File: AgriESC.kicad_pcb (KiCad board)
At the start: 2 copper layers, 91.9 x 64 mm, 312 parts, among them J1 SUPPLY, J10 GPIO, J11 USB_OTG, J12 HALL_ENC, J2 PH_A, J3 PH_B, J4 PH_C, J6 COMM, J7 SERVO, J8 CAN, J9 SWD, SW1 SW_SPDT, U1 FDMS7698, U10 STM32F405RGT6, U11 DRV8303, U12 TJA1051TK-3, U13 LMR16006YQ, U14 MCP1700-3302E_SOT23, U15 MCP1700-3302E_SOT23, U2 FDMS7698, U3 FDMS7698, U4 FDMS7698, U5 FDMS7698, U6 FDMS7698, U7 MAX9920, U8 MAX9920, U9 MAX9920, Y1 8M Resonator

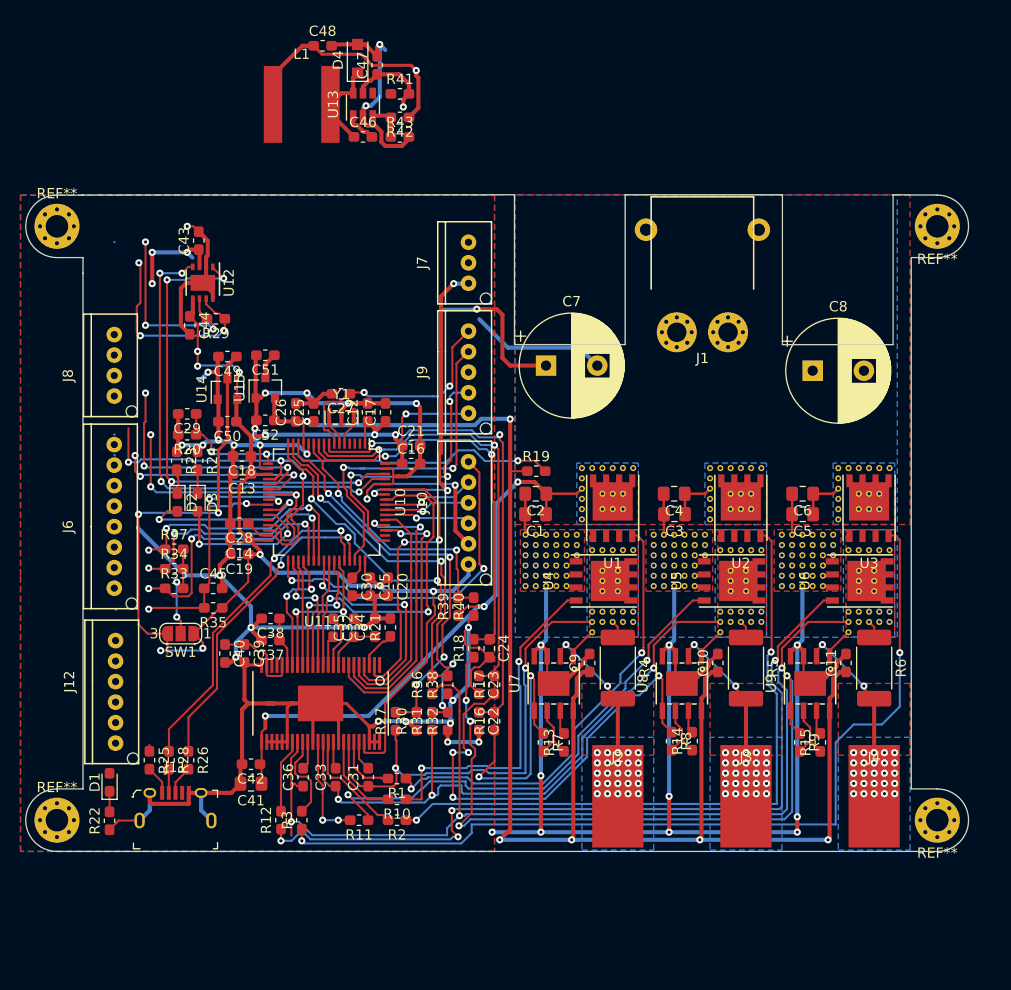
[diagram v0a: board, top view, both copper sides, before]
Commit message: Version 1.0 completed
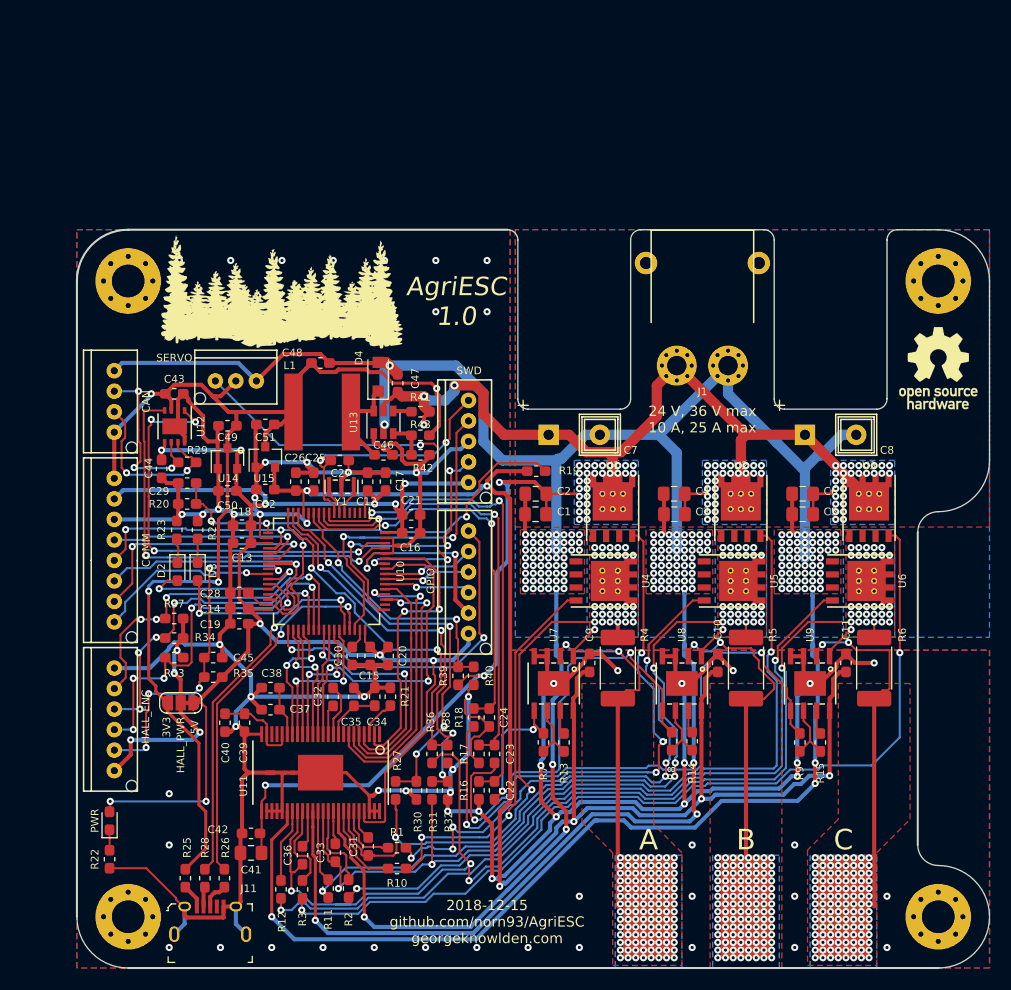
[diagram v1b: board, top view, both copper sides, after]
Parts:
- removed D1: BLUE, LED_SMD:LED_0603_1608Metric_Pad1.05x0.95mm_HandSolder
- removed J10: GPIO, AgriESC:JST_PA_01x06
- removed J12: HALL_ENC, AgriESC:JST_PA_01x06
- removed J4: PH_C, Connector_Wire:SolderWirePad_1x01_SMD_5x10mm
- removed J6: COMM, AgriESC:JST_PA_01x08
- removed J7: SERVO, AgriESC:JST_PA_01x03
- removed J8: CAN, AgriESC:JST_PA_01x04
- removed J9: SWD, AgriESC:JST_PA_01x05
- removed the REF** at (194.9, 64.7)
- removed the REF** at (188.2, 103.2)
- removed the REF** at (172.8, 91.2)
- removed the REF** at (172.8, 90.2)
- removed the REF** at (172.8, 89.2)
- removed the REF** at (172.8, 88.2)
- removed the REF** at (173.8, 88.2)
- removed the REF** at (174.8, 88.2)
- removed the REF** at (175.8, 88.2)
- removed the REF** at (176.8, 88.2)
- removed the REF** at (177.8, 88.2)
- removed the REF** at (177.8, 103.2)
- removed the REF** at (188.2, 102.2)
- removed the REF** at (176.8, 103.2)
- removed the REF** at (175.8, 103.2)
- removed the REF** at (174.8, 103.2)
- removed the REF** at (173.8, 104.2)
- removed the REF** at (173.8, 103.2)
- removed the REF** at (173.8, 102.2)
- removed the REF** at (174.8, 102.2)
- removed the REF** at (175.8, 102.2)
- removed the REF** at (176.8, 102.2)
- removed the REF** at (177.8, 102.2)
- removed the REF** at (189.2, 103.2)
- removed the REF** at (177.8, 96.2)
- removed the REF** at (176.8, 96.2)
- removed the REF** at (175.8, 96.2)
- removed the REF** at (174.8, 96.2)
- removed the REF** at (173.8, 96.2)
- removed the REF** at (165.2, 88.2)
- removed the REF** at (164.2, 88.2)
- removed the REF** at (163.2, 88.2)
- removed the REF** at (162.2, 88.2)
- removed the REF** at (161.2, 88.2)
- removed the REF** at (189.2, 102.2)
- removed the REF** at (160.2, 88.2)
- removed the REF** at (160.2, 89.2)
- removed the REF** at (160.2, 90.2)
- removed the REF** at (160.2, 91.2)
- removed the REF** at (160.2, 92.2)
- removed the REF** at (160.2, 93.2)
- removed the REF** at (158.8, 99.8)
- removed the REF** at (157.8, 99.8)
- removed the REF** at (156.8, 99.8)
- removed the REF** at (155.8, 99.8)
- removed the REF** at (190.2, 103.2)
- removed the REF** at (154.8, 99.8)
- removed the REF** at (158.8, 98.8)
- removed the REF** at (157.8, 98.8)
- removed the REF** at (156.8, 98.8)
- removed the REF** at (155.8, 98.8)
- removed the REF** at (154.8, 98.8)
- removed the REF** at (158.8, 97.8)
- removed the REF** at (157.8, 97.8)
- removed the REF** at (156.8, 97.8)
- removed the REF** at (155.8, 97.8)
- removed the REF** at (190.2, 102.2)
- removed the REF** at (154.8, 97.8)
- removed the REF** at (158.8, 96.8)
- removed the REF** at (157.8, 96.8)
- removed the REF** at (156.8, 96.8)
- removed the REF** at (155.8, 96.8)
- removed the REF** at (154.8, 96.8)
- removed the REF** at (159.8, 95.8)
- removed the REF** at (158.8, 95.8)
- removed the REF** at (157.8, 95.8)
- removed the REF** at (156.8, 95.8)
- removed the REF** at (190.2, 96.2)
- removed the REF** at (155.8, 95.8)
- removed the REF** at (154.8, 95.8)
- removed the REF** at (159.8, 94.8)
- removed the REF** at (158.8, 94.8)
- removed the REF** at (157.8, 94.8)
- removed the REF** at (156.8, 94.8)
- removed the REF** at (155.8, 94.8)
- removed the REF** at (154.8, 94.8)
- removed the REF** at (165.2, 103.2)
- removed the REF** at (164.2, 103.2)
- removed the REF** at (189.2, 96.2)
- removed the REF** at (163.2, 103.2)
- removed the REF** at (162.2, 103.2)
- removed the REF** at (161.2, 104.2)
- removed the REF** at (161.2, 103.2)
- removed the REF** at (161.2, 102.2)
- removed the REF** at (165.2, 102.2)
- removed the REF** at (164.2, 102.2)
- removed the REF** at (163.2, 102.2)
- removed the REF** at (162.2, 102.2)
- removed the REF** at (165.2, 96.2)
- removed the REF** at (188.2, 96.2)
- removed the REF** at (164.2, 96.2)
- removed the REF** at (163.2, 96.2)
- removed the REF** at (162.2, 96.2)
- removed the REF** at (161.2, 96.2)
- removed the REF** at (109.1, 64.7)
- removed the REF** at (187.2, 96.2)
- removed the REF** at (194.9, 122.6)
- removed the REF** at (186.2, 96.2)
- removed the REF** at (190.2, 88.2)
- removed the REF** at (189.2, 88.2)
- removed the REF** at (188.2, 88.2)
- removed the REF** at (187.2, 88.2)
- removed the REF** at (186.2, 88.2)
- removed the REF** at (185.2, 93.2)
- removed the REF** at (185.2, 92.2)
- removed the REF** at (185.2, 91.2)
- removed the REF** at (185.2, 90.2)
- removed the REF** at (109.1, 122.6)
- removed the REF** at (185.2, 89.2)
- removed the REF** at (185.2, 88.2)
- removed the REF** at (183.8, 99.8)
- removed the REF** at (182.8, 99.8)
- removed the REF** at (181.8, 99.8)
- removed the REF** at (180.8, 99.8)
- removed the REF** at (179.8, 99.8)
- removed the REF** at (183.8, 98.8)
- removed the REF** at (182.8, 98.8)
- removed the REF** at (181.8, 98.8)
- removed the REF** at (159.8, 96.8)
- removed the REF** at (180.8, 98.8)
- removed the REF** at (179.8, 98.8)
- removed the REF** at (183.8, 97.8)
- removed the REF** at (182.8, 97.8)
- removed the REF** at (181.8, 97.8)
- removed the REF** at (180.8, 97.8)
- removed the REF** at (179.8, 97.8)
- removed the REF** at (184.8, 96.8)
- removed the REF** at (183.8, 96.8)
- removed the REF** at (182.8, 96.8)
- removed the REF** at (186.2, 104.2)
- removed the REF** at (181.8, 96.8)
- removed the REF** at (180.8, 96.8)
- removed the REF** at (179.8, 96.8)
- removed the REF** at (184.8, 95.8)
- removed the REF** at (183.8, 95.8)
- removed the REF** at (182.8, 95.8)
- removed the REF** at (181.8, 95.8)
- removed the REF** at (180.8, 95.8)
- removed the REF** at (179.8, 95.8)
- removed the REF** at (184.8, 94.8)
- removed the REF** at (186.2, 103.2)
- removed the REF** at (183.8, 94.8)
- removed the REF** at (182.8, 94.8)
- removed the REF** at (181.8, 94.8)
- removed the REF** at (180.8, 94.8)
- removed the REF** at (179.8, 94.8)
- removed the REF** at (171.2, 99.8)
- removed the REF** at (170.2, 99.8)
- removed the REF** at (169.2, 99.8)
- removed the REF** at (168.2, 99.8)
- removed the REF** at (167.2, 99.8)
- removed the REF** at (186.2, 102.2)
- removed the REF** at (171.2, 98.8)
- removed the REF** at (170.2, 98.8)
- removed the REF** at (169.2, 98.8)
- removed the REF** at (168.2, 98.8)
- removed the REF** at (167.2, 98.8)
- removed the REF** at (171.2, 97.8)
- removed the REF** at (170.2, 97.8)
- removed the REF** at (169.2, 97.8)
- removed the REF** at (168.2, 97.8)
- removed the REF** at (167.2, 97.8)
- removed the REF** at (187.2, 103.2)
- removed the REF** at (172.2, 96.8)
- removed the REF** at (171.2, 96.8)
- removed the REF** at (170.2, 96.8)
- removed the REF** at (169.2, 96.8)
- removed the REF** at (168.2, 96.8)
- removed the REF** at (167.2, 96.8)
- removed the REF** at (172.2, 95.8)
- removed the REF** at (171.2, 95.8)
- removed the REF** at (170.2, 95.8)
- removed the REF** at (169.2, 95.8)
- removed the REF** at (187.2, 102.2)
- removed the REF** at (168.2, 95.8)
- removed the REF** at (167.2, 95.8)
- removed the REF** at (172.2, 94.8)
- removed the REF** at (171.2, 94.8)
- removed the REF** at (170.2, 94.8)
- removed the REF** at (169.2, 94.8)
- removed the REF** at (168.2, 94.8)
- removed the REF** at (167.2, 94.8)
- removed the REF** at (172.8, 93.2)
- removed the REF** at (172.8, 92.2)
- removed SW1: SW_SPDT, Jumper:SolderJumper-3_P1.3mm_Open_RoundedPad1.0x1.5mm_NumberLabels
- added C: PH_C, Connector_Wire:SolderWirePad_1x01_SMD_5x10mm, F.Cu at (185.8, 131.0)
- added CAN: CAN, AgriESC:JST_PA_01x04, F.Cu at (114.6, 82.8)
- added COMM: COMM, AgriESC:JST_PA_01x08, F.Cu at (114.6, 97.2)
- added G***: LOGO3, AgriESC:LOGO3, F.Cu at (131.0, 71.0)
- added GPIO: GPIO, AgriESC:JST_PA_01x06, F.Cu at (149.2, 98.4)
- added HALL_ENC: HALL_ENC, AgriESC:JST_PA_01x06, F.Cu at (114.7, 111.8)
- added HALL_PWR: SW_SPDT, Jumper:SolderJumper-3_P1.3mm_Open_RoundedPad1.0x1.5mm_NumberLabels, F.Cu at (121.1, 111.1)
- added NT1: Net-Tie_2, NetTie:NetTie-2_SMD_Pad0.5mm, B.Cu at (157.8, 106.0)
- added NT2: Net-Tie_2, NetTie:NetTie-2_SMD_Pad0.5mm, B.Cu at (170.2, 106.0)
- added NT3: Net-Tie_2, NetTie:NetTie-2_SMD_Pad0.5mm, B.Cu at (182.8, 106.0)
- added PWR: BLUE, LED_SMD:LED_0603_1608Metric_Pad1.05x0.95mm_HandSolder, F.Cu at (114.2, 122.6)
- added REF**: MountingHole_3.2mm_M3_Pad_Via, MountingHole:MountingHole_3.2mm_M3_Pad_Via, F.Cu at (116.0, 132.0)
- added REF**: MountingHole_3.2mm_M3_Pad_Via, MountingHole:MountingHole_3.2mm_M3_Pad_Via, F.Cu at (195.0, 70.0)
- added REF**: MountingHole_3.2mm_M3_Pad_Via, MountingHole:MountingHole_3.2mm_M3_Pad_Via, F.Cu at (195.0, 132.0)
- added REF**: MountingHole_3.2mm_M3_Pad_Via, MountingHole:MountingHole_3.2mm_M3_Pad_Via, F.Cu at (116.0, 70.0)
- added REF**: OSHW-Logo_7.5x8mm_SilkScreen, Symbol:OSHW-Logo_7.5x8mm_SilkScreen, F.Cu at (195.0, 78.5)
- added SERVO: SERVO, AgriESC:JST_PA_01x03, F.Cu at (126.5, 79.8)
- added SWD: SWD, AgriESC:JST_PA_01x05, F.Cu at (149.2, 85.6)
- C7, C8: footprint Capacitor_THT:CP_Radial_D10.0mm_P5.00mm -> AgriESC:CP_Radial_D10.0mm_P5.00mm_Side_Mounted
- moved U13 31.1 mm to (140.9, 83.8)
- moved C46 31.1 mm to (140.9, 87.0)
- moved C47 31.1 mm to (142.3, 80.0)
- moved D4 31.1 mm to (140.4, 79.3)
- moved R41 31.1 mm to (144.5, 82.8)
- moved R42 31.1 mm to (144.5, 85.0)
- moved R43 31.1 mm to (144.5, 87.0)
- moved C48 30.9 mm to (134.8, 78.0)
- moved L1 30.1 mm to (134.9, 82.8)
- moved C43 15.1 mm to (120.5, 81.0), turned to 0 degrees
- moved R29 14.3 mm to (121.8, 87.7)
- moved C44 14.3 mm to (119.3, 88.3)
- moved U12 14.3 mm to (120.5, 84.2)
- moved R25 12.0 mm to (121.6, 128.2)
- moved R26 12.0 mm to (125.4, 128.2)
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- renumbered J2 to A, J3 to B
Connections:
- C1 pad 2: SL_A -> GND
- C10 pad 2: SL_A -> GND
- C11 pad 2: SL_A -> GND
- C12 pad 2: SL_A -> GND
- C13 pad 2: SL_A -> GND
- C14 pad 2: SL_A -> GND
- C15 pad 2: SL_A -> GND
- C16 pad 2: SL_A -> GND
- C17 pad 2: SL_A -> GND
- C18 pad 2: SL_A -> GND
- C19 pad 2: SL_A -> GND
- C2 pad 2: SL_A -> GND
- C20 pad 2: SL_A -> GND
- C21 pad 2: SL_A -> GND
- C22 pad 2: SL_A -> GND
- C23 pad 2: SL_A -> GND
- C24 pad 2: SL_A -> GND
- C25 pad 2: SL_A -> GND
- C26 pad 2: SL_A -> GND
- C27 pad 2: SL_A -> GND
- C28 pad 2: SL_A -> GND
- C29 pad 2: SL_A -> GND
- C3 pad 2: SL_A -> GND
- C30 pad 2: SL_A -> GND
- C34 pad 2: SL_A -> GND
- C35 pad 2: SL_A -> GND
- C37 pad 2: SL_A -> GND
- C38 pad 2: SL_A -> GND
- C39 pad 2: SL_A -> GND
- C4 pad 2: SL_A -> GND
- C40 pad 2: SL_A -> GND
- C41 pad 2: SL_A -> GND
- C42 pad 2: SL_A -> GND
- C43 pad 2: SL_A -> GND
- C44 pad 2: SL_A -> GND
- C45 pad 2: SL_A -> GND
- C47 pad 2: SL_A -> GND
- C48 pad 2: SL_A -> GND
- C49 pad 2: SL_A -> GND
- C5 pad 2: SL_A -> GND
- C50 pad 2: SL_A -> GND
- C51 pad 2: SL_A -> GND
- C52 pad 2: SL_A -> GND
- C6 pad 2: SL_A -> GND
- C7 pad 2: SL_A -> GND
- C8 pad 2: SL_A -> GND
- C9 pad 2: SL_A -> GND
- D4 pad 2: SL_A -> GND
- J1 pad 1: SL_A -> GND
- J11 pad 5: SL_A -> GND
- J11 pad 6: SL_A -> GND
- R20 pad 2: SL_A -> GND
- R21 pad 2: SL_A -> GND
- R22 pad 1: SL_A -> GND
- R23 pad 1: SL_A -> GND
- R24 pad 1: SL_A -> GND
- R30 pad 1: SL_A -> GND
- R32 pad 1: SL_A -> GND
- R33 pad 2: Net-(J12-Pad6) -> VCC
- R34 pad 2: Net-(J12-Pad6) -> VCC
- R37 pad 2: Net-(J12-Pad6) -> VCC
- R38 pad 1: SL_A -> GND
- R40 pad 1: SL_A -> GND
- R43 pad 2: SL_A -> GND
- U10 pad 12: SL_A -> GND
- U10 pad 18: SL_A -> GND
- U10 pad 60: SL_A -> GND
- U10 pad 63: SL_A -> GND
- U11 pad 24: SL_A -> GND
- U11 pad 26: SL_A -> GND
- U11 pad 27: SL_A -> GND
- U11 pad 28: SL_A -> GND
- U11 pad 29: SL_A -> GND
- U11 pad 30: SL_A -> SL_C
- U11 pad 35: SL_A -> SL_B
- U11 pad 46: SL_A -> GND
- U11 pad 47: SL_A -> GND
- U11 pad 48: SL_A -> GND
- U12 pad 2: SL_A -> GND
- U12 pad 8: SL_A -> GND
- U12 pad 9: SL_A -> GND
- U13 pad 2: SL_A -> GND
- U14 pad 1: SL_A -> GND
- U15 pad 1: SL_A -> GND
- U4 pad 3: SL_A -> GND
- U5 pad 3: SL_A -> GND
- U6 pad 3: SL_A -> GND
- U7 pad 3: SL_A -> GND
- U7 pad 4: SL_A -> GND
- U8 pad 3: SL_A -> GND
- U8 pad 4: SL_A -> GND
- U9 pad 3: SL_A -> GND
- U9 pad 4: SL_A -> GND
- Y1 pad 2: SL_A -> GND
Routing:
- net GND: track 0.00 -> 575.2 mm, vias 0 -> 235
- net SL_A: track 467.1 -> 53.6 mm, vias 38 -> 3
- net SL_C: track 0.00 -> 84.5 mm, vias 0 -> 3
- net SL_B: track 0.00 -> 69.9 mm, vias 0 -> 3
- net SUPPLY: track 92.2 -> 153.9 mm, vias 5 -> 90
- net VCC: track 135.5 -> 190.3 mm, vias 12 -> 15
- net +5V: track 77.2 -> 113.8 mm, vias 6 -> 4
- net Net-(J3-Pad1): track 19.7 -> 36.6 mm, vias 27 -> 114
- net Net-(J2-Pad1): track 18.3 -> 34.1 mm, vias 27 -> 114
- net Net-(J4-Pad1): track 19.3 -> 34.2 mm, vias 27 -> 114
- net SH_B: track 66.1 -> 80.4 mm, vias 3 -> 35
- net SERVO: track 31.0 -> 44.2 mm
- net C_A: track 26.2 -> 13.0 mm
- net Net-(R1-Pad1): track 43.8 -> 56.3 mm, vias 2 -> 6
- net Net-(R11-Pad1): track 49.2 -> 61.5 mm, vias 2 -> 4
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- added copper zone on B.Cu, net GND
- added copper zone on F.Cu, net GND
- removed copper zone on B.Cu, net SL_A
- removed copper zone on F.Cu, net SL_A
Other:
- board size 91.9 x 64 mm -> 89 x 72 mm
- board text added: "2018-12-15 github.com/norn93/AgriESC georgeknowlden.com"
- board text added: "24 V, 36 V max 10 A, 25 A max"
- board text added: "AgriESC 1.0"
